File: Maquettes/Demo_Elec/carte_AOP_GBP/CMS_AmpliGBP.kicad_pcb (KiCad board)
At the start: 2 copper layers, 49.2 x 27.8 mm, 7 parts, among them J1 Conn_01x18, U1 TL084

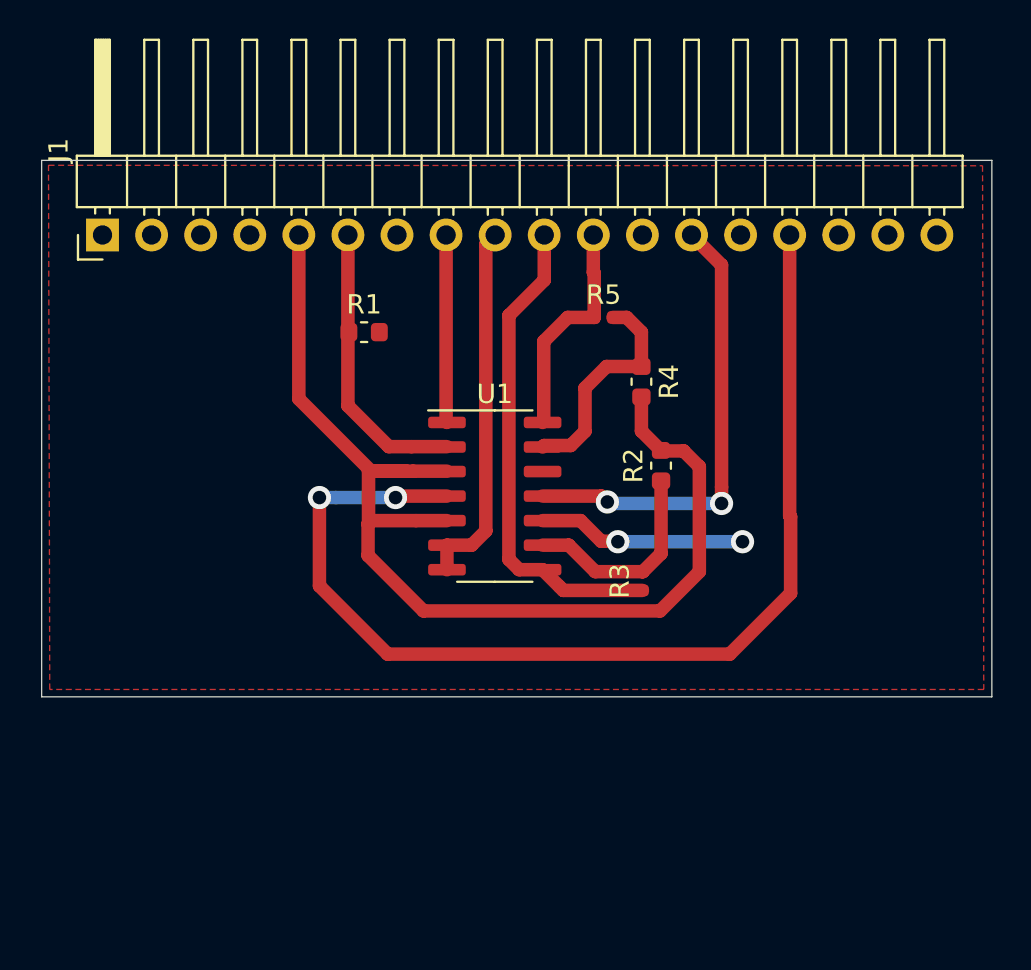
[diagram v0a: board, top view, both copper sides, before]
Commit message: Amplifier Demo Board
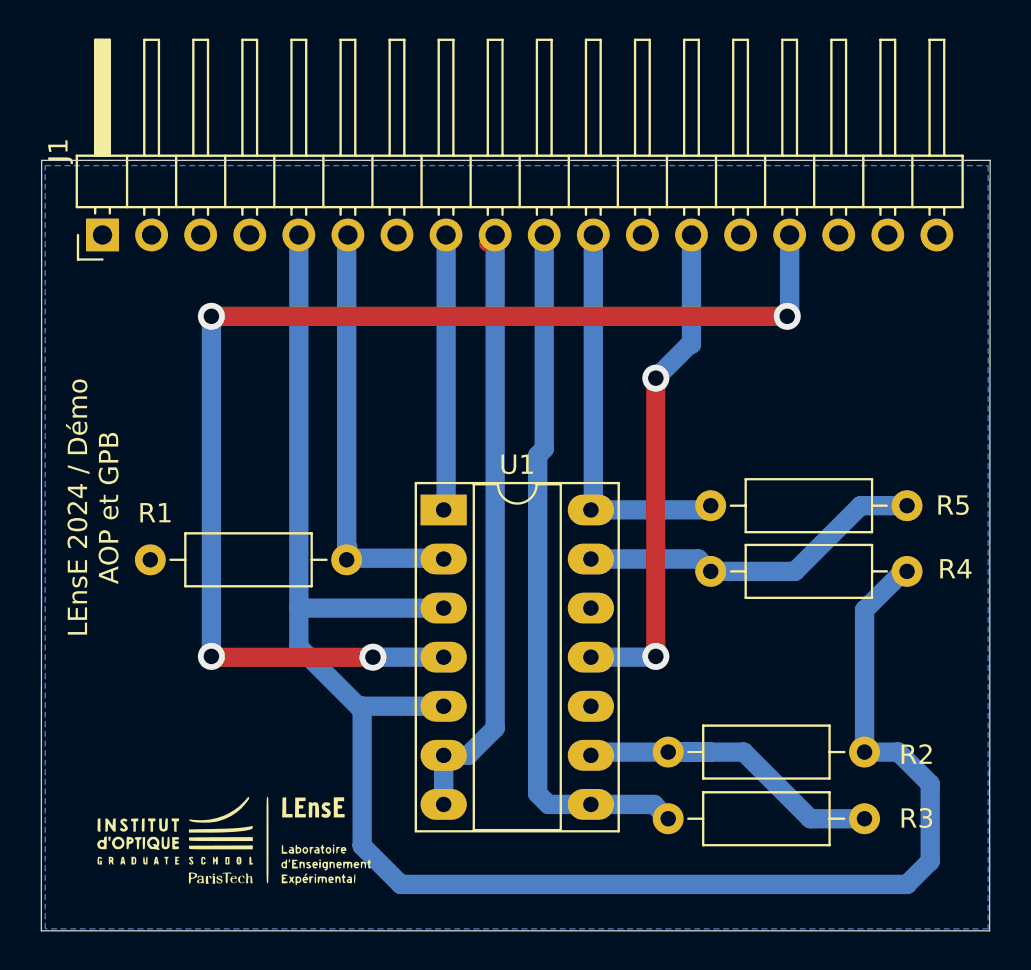
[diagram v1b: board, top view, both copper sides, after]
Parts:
- added G***: LOGO, LEnsE_devices:Logo_Small, F.Cu at (133.2, 128.9)
- R1, R2, R4: footprint Resistor_SMD:R_0603_1608Metric -> Resistor_THT:R_Axial_DIN0207_L6.3mm_D2.5mm_P10.16mm_Horizontal
- R3, R5: footprint Resistor_SMD:R_0402_1005Metric -> Resistor_THT:R_Axial_DIN0207_L6.3mm_D2.5mm_P10.16mm_Horizontal
- U1: footprint Package_SO:SOIC-14_3.9x8.7mm_P1.27mm -> Package_DIP:DIP-14_W7.62mm_Socket_LongPads
- moved R2 14.8 mm to (155.6, 124.5), turned to 0 degrees
- moved R3 12.4 mm to (155.6, 128.0), turned to 0 degrees
- moved R1 11.8 mm to (139.0, 114.6), turned to 180 degrees
- moved R5 11.2 mm to (157.8, 111.8)
- moved R4 10.4 mm to (157.8, 115.2), turned to 0 degrees
- moved U1 2.74 mm to (144.0, 112.0)
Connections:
- J1 pad 1: Net-(J1-Pad1) -> unconnected-(J1-Pin_1-Pad1)
- J1 pad 2: Net-(J1-Pad2) -> unconnected-(J1-Pin_2-Pad2)
- J1 pad 3: Net-(J1-Pad3) -> unconnected-(J1-Pin_3-Pad3)
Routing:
- net IN1: track 58.3 -> 94.0 mm
- net OUT2: track 19.1 -> 32.0 mm
- net OUT3: track 25.1 -> 36.3 mm
- net GND: track 10.8 -> 0.00 mm, vias 2 -> 0
- net OUT4: track 11.6 -> 20.6 mm
- net Net-(U1C--): track 10.8 -> 17.9 mm
- net +15V: track 56.9 -> 63.9 mm, vias 2 -> 4
- net IN2: track 14.8 -> 21.3 mm
- net Net-(U1D--): track 11.7 -> 18.0 mm
- net OUT1: track 9.72 -> 14.3 mm
- net -15V: track 24.0 -> 26.0 mm
- added copper zone on B.Cu, net GND
- removed copper zone on F.Cu, net GND
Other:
- board size 49.2 x 27.8 mm -> 49.1 x 39.9 mm
- board text added: "LEnsE 2024 / Démo AOP et GPB"
